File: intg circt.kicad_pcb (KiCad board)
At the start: 4 copper layers, 18.2 x 40.8 mm, 55 parts, among them J1 Conn_01x01_Pin, J2 USB_C_Receptacle_USB2.0_16P, J3 Conn_01x02_Pin, J4 5033981892, J5 Conn_01x02_Pin, J6 Conn_01x01_Pin, U1 ESP32-S3-MINI-1U, U2 MAXM86161EFD_T, U3 BMI270, U4 BQ24074RGT, U6 USBLC6-2P6, U7 MAX17048X+T10, U8 TLV75533PDBV, U9 LMV358IDR

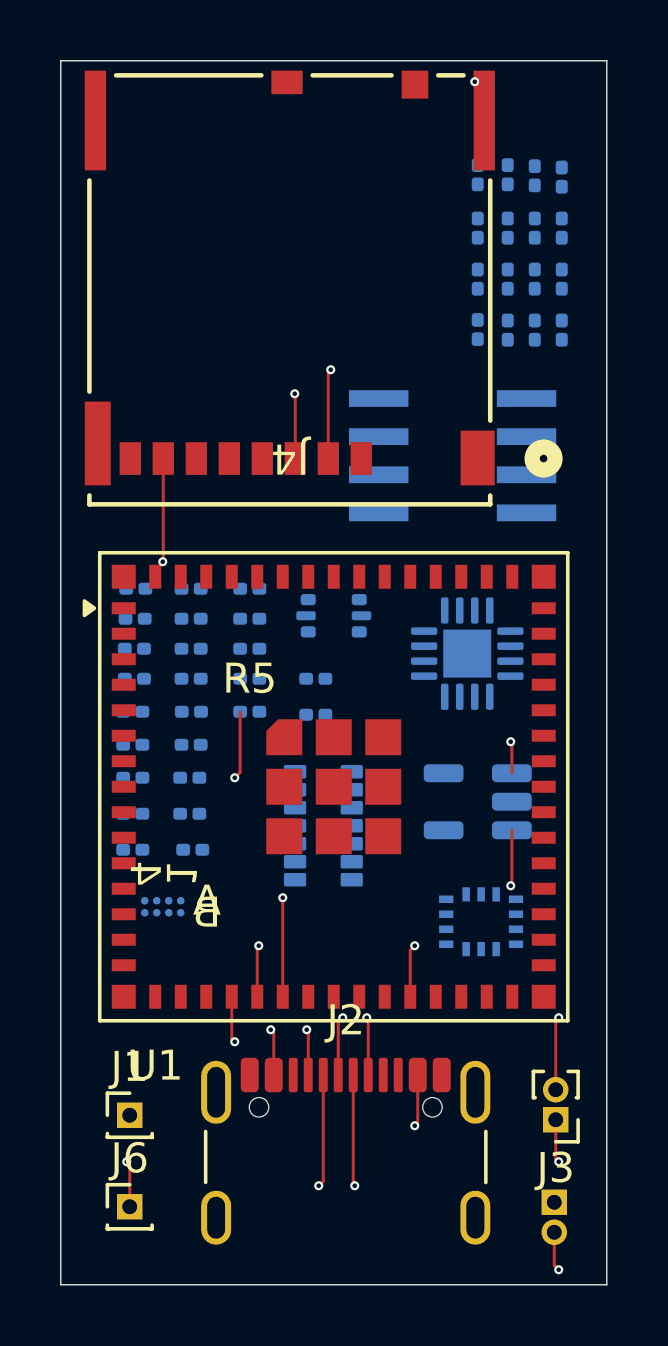
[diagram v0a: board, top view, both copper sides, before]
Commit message: done
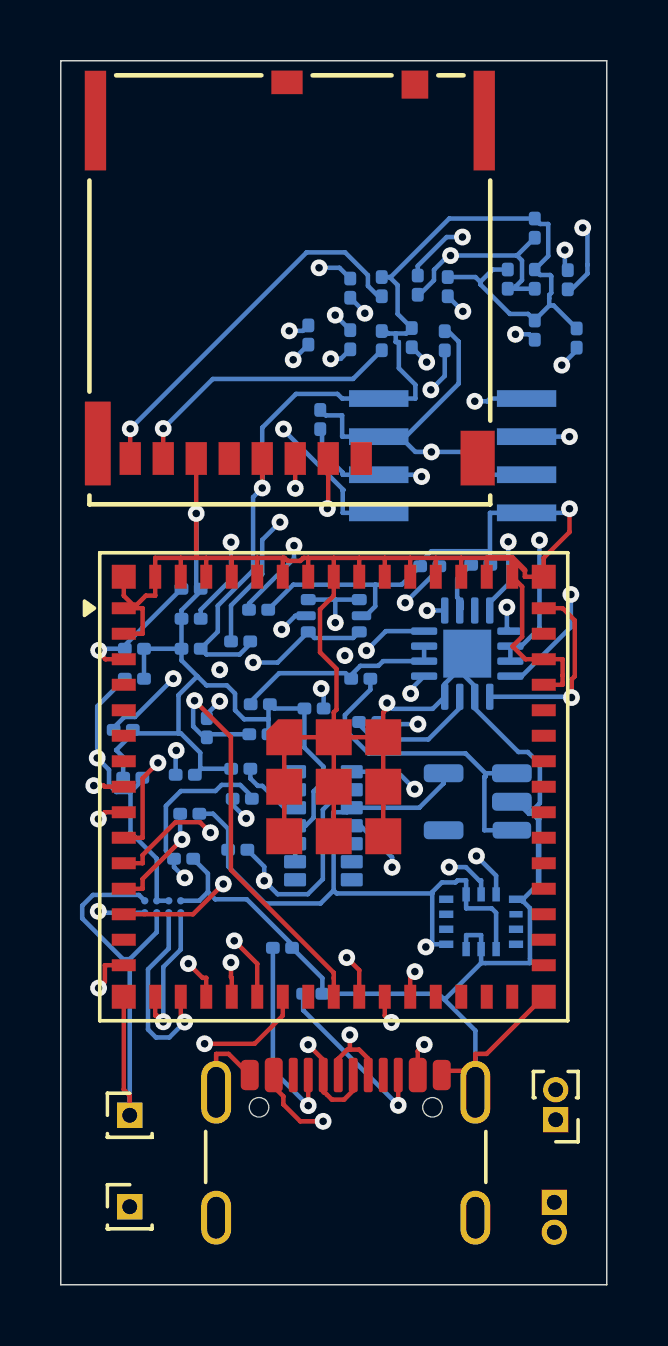
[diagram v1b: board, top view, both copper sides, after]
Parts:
- moved R7 8.49 mm to (76.2, 56.8)
- moved R6 7.95 mm to (75.2, 55.3)
- moved R18 7.60 mm to (77.5, 35.0)
- moved R1 7.43 mm to (81.8, 42.5)
- moved R14 7.08 mm to (78.5, 35.0)
- moved C1 6.95 mm to (73.8, 49.3)
- moved R20 6.68 mm to (76.1, 34.8)
- moved C2 6.67 mm to (76.2, 47.3)
- moved TH1 6.60 mm to (80.1, 42.5)
- moved C16 6.26 mm to (80.6, 35.0)
- moved R19 6.05 mm to (76.5, 37.7)
- moved C12 6.01 mm to (71.9, 52.3)
- moved R11 6.01 mm to (73.8, 50.3)
- moved R15 6.01 mm to (78.5, 33.2)
- moved R17 5.62 mm to (77.5, 33.3)
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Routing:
- net GND: track 0.00 -> 206.9 mm, vias 0 -> 5
- net +3V3: track 17.4 -> 146.1 mm, vias 2 -> 5
- net /U1_BAT: track 0.00 -> 48.0 mm, vias 0 -> 2
- net /OUT_A: track 0.00 -> 43.7 mm, vias 0 -> 5
- net /OUT_B: track 0.00 -> 36.9 mm, vias 0 -> 2
- net /VBUS: track 11.3 -> 47.3 mm, vias 4 -> 6
- net /~{CE}: track 0.00 -> 30.7 mm, vias 0 -> 2
- net Net-(U9-INB+): track 0.00 -> 21.8 mm, vias 0 -> 4
- net /U3_SCX: track 0.00 -> 18.9 mm, vias 0 -> 2
- net /D+: track 5.50 -> 23.9 mm, vias 6 -> 3
- net /D-: track 8.66 -> 26.4 mm, vias 2 -> 4
- net /~{CHG}: track 0.00 -> 16.7 mm, vias 0 -> 2
- net /U3_SDX: track 0.00 -> 16.5 mm, vias 0 -> 2
- net /U2_SDA: track 0.00 -> 14.8 mm, vias 0 -> 2
- net /USB_D-: track 0.00 -> 14.7 mm, vias 0 -> 1
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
